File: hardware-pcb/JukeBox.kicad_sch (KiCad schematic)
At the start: 77 parts, among them J1 USB4105-GF-A, J2 AudioJack4_Ground, Q1 Q_NPN_ECB, SW1 SW_SPST, SW10 SW_SPST, SW11 SW_SPST, SW12 SW_SPST, SW2 SW_SPST, SW3 SW_SPST, SW4 SW_SPST, SW5 SW_SPST, SW6 SW_SPST, SW7 SW_SPST, SW8 SW_SPST, SW9 SW_SPST, U1 NCP1117-3.3_SOT223, U2 W25Q128JVS, U3 RP2040, U4 st7789v, Y1 ECS-120-20-33-AEL-TR

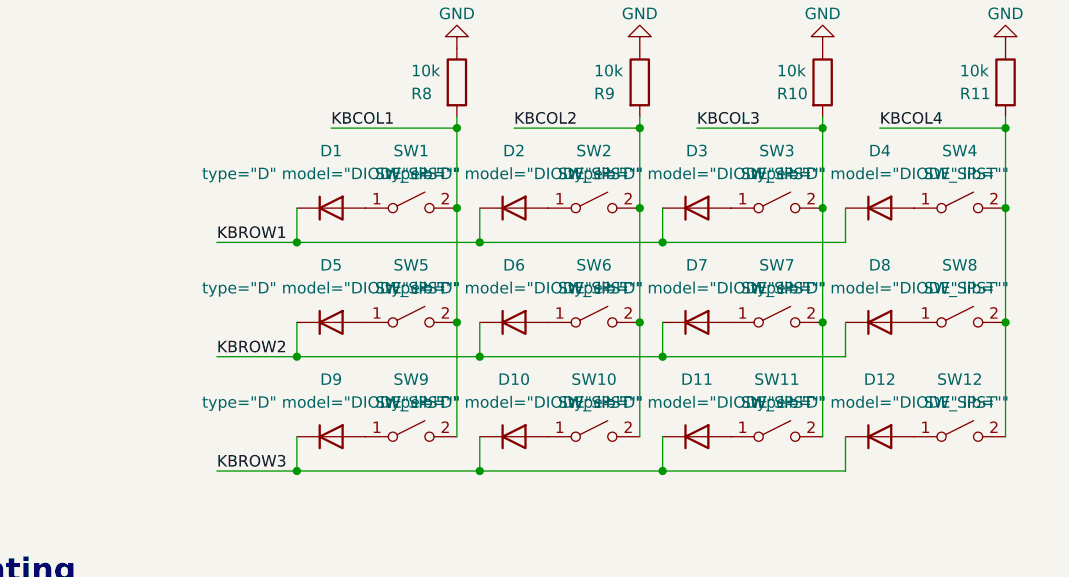
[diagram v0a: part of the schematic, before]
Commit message: minor updates for production
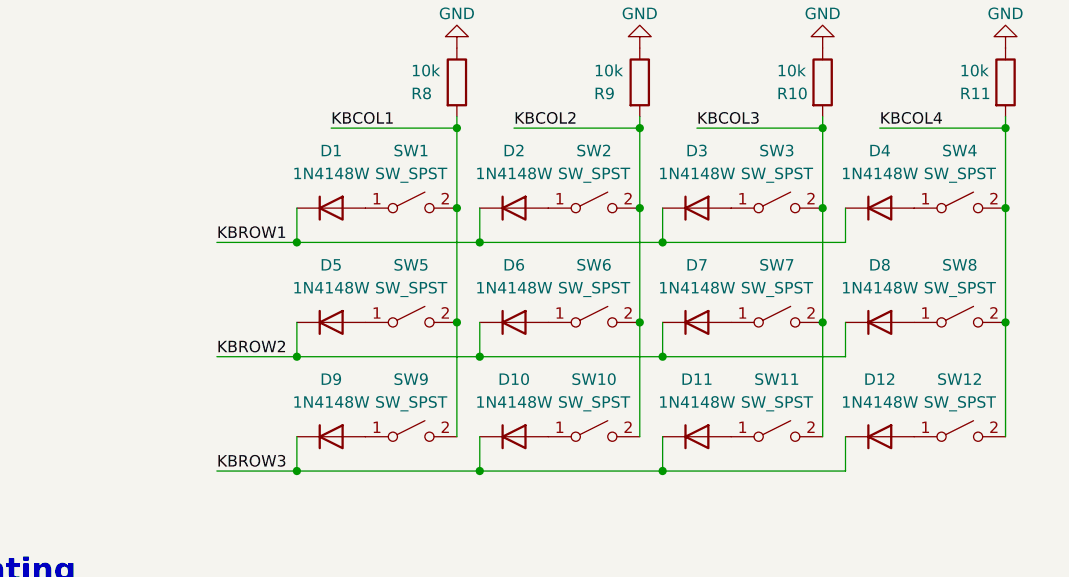
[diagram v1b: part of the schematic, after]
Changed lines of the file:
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@@
 			)
 		)
-		(property "Sim.Params" "type=\"D\" model=\"DIODE\" lib=\"\""
+		(property "Sim.Params" "1N4148W"
 			(at 0 0 0)
 			(effects
@@
 			)
 		)
-		(property "Sim.Params" "type=\"D\" model=\"DIODE\" lib=\"\""
+		(property "Sim.Params" "1N4148W"
 			(at 0 0 0)
 			(effects
@@
 			)
 		)
-		(property "Sim.Params" "type=\"D\" model=\"DIODE\" lib=\"\""
+		(property "Sim.Params" "1N4148W"
 			(at 0 0 0)
 			(effects
@@
 			)
 		)
-		(property "Sim.Params" "type=\"D\" model=\"DIODE\" lib=\"\""
+		(property "Sim.Params" "1N4148W"
 			(at 0 0 0)
 			(effects
@@
 			)
 		)
-		(property "Sim.Params" "type=\"D\" model=\"DIODE\" lib=\"\""
+		(property "Sim.Params" "1N4148W"
 			(at 0 0 0)
 			(effects
@@
 			)
 		)
-		(property "Sim.Params" "type=\"D\" model=\"DIODE\" lib=\"\""
+		(property "Sim.Params" "1N4148W"
 			(at 0 0 0)
 			(effects
@@
 			)
 		)
-		(property "Sim.Params" "type=\"D\" model=\"DIODE\" lib=\"\""
+		(property "Sim.Params" "1N4148W"
 			(at 0 0 0)
 			(effects
@@
 			)
 		)
-		(property "Sim.Params" "type=\"D\" model=\"DIODE\" lib=\"\""
+		(property "Sim.Params" "1N4148W"
 			(at 0 0 0)
 			(effects
@@
 			)
 		)
-		(property "Sim.Params" "type=\"D\" model=\"DIODE\" lib=\"\""
+		(property "Sim.Params" "1N4148W"
 			(at 0 0 0)
 			(effects
@@
 			)
 		)
-		(property "Sim.Params" "type=\"D\" model=\"DIODE\" lib=\"\""
+		(property "Sim.Params" "1N4148W"
 			(at 0 0 0)
 			(effects
@@
 			)
 		)
-		(property "Sim.Params" "type=\"D\" model=\"DIODE\" lib=\"\""
+		(property "Sim.Params" "1N4148W"
 			(at 0 0 0)
 			(effects
@@
 			)
 		)
-		(property "Sim.Params" "type=\"D\" model=\"DIODE\" lib=\"\""
+		(property "Sim.Params" "1N4148W"
 			(at 0 0 0)
 			(effects
